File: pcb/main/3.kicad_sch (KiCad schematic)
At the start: 10 parts

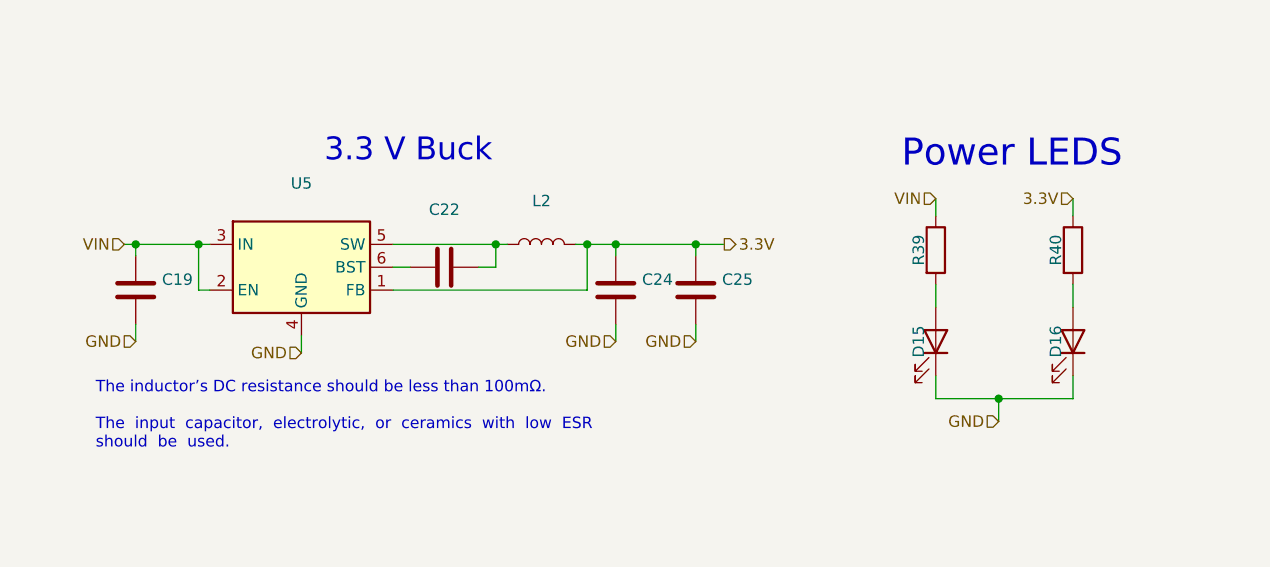
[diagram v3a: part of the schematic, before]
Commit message: feat: updated BOM
BOM ready to order in v0.2
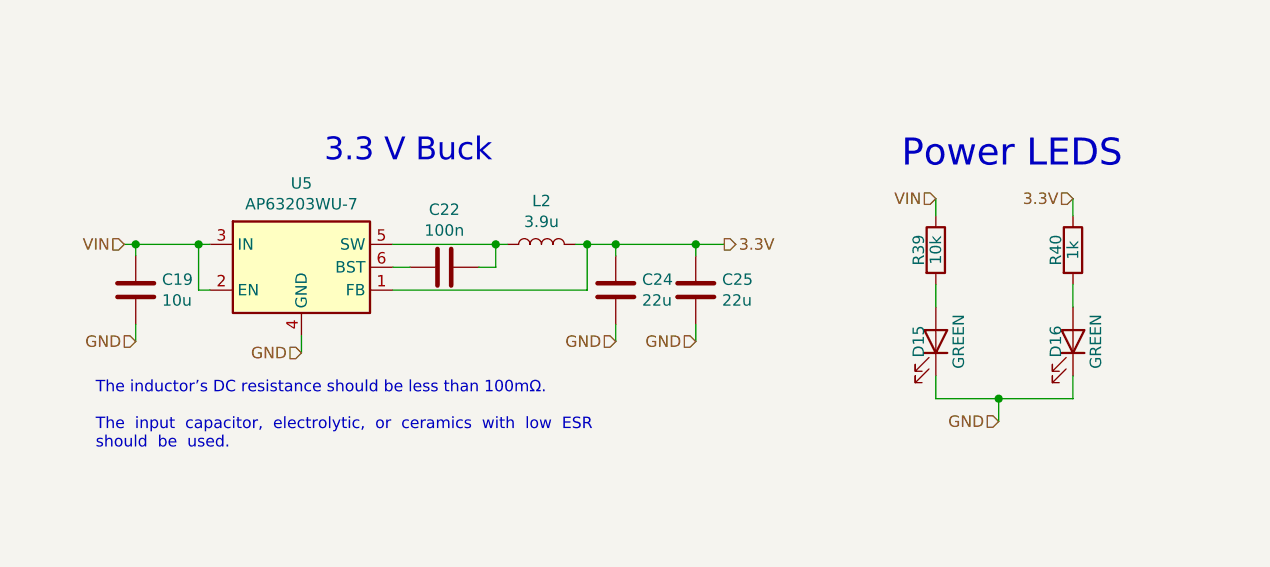
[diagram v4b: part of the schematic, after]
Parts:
- C19: value (none) -> 10u; footprint (none) -> Capacitor_SMD:C_0805_2012Metric_Pad1.18x1.45mm_HandSolder; MFN Wurth Elektronik -> Samsung Electro-Mechanics; MFP 885012207072 -> CL21A106KOQNNNG; S1PL https://www.mouser.com/ProductDetail/Wurth-Elektronik/88501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 -> https://www.mouser.com/ProductDetail/Samsung-Electro-Mechan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; S1PN 710-885012207072 -> 187-CL21A106KOQNNNG
- C22: value (none) -> 100n; footprint (none) -> Capacitor_SMD:C_0805_2012Metric_Pad1.18x1.45mm_HandSolder
- C24, C25: value (none) -> 22u; footprint (none) -> Capacitor_SMD:C_0805_2012Metric_Pad1.15x1.40mm_HandSolder
- D15, D16: value (none) -> GREEN; footprint (none) -> LED_SMD:LED_0805_2012Metric_Pad1.15x1.40mm_HandSolder
- L2: value (none) -> 3.9u; footprint (none) -> Inductor_SMD:L_Taiyo-Yuden_NR-24xx_HandSoldering
- R39: value (none) -> 10k; footprint (none) -> Resistor_SMD:R_0805_2012Metric_Pad1.20x1.40mm_HandSolder
- R40: value (none) -> 1k; footprint (none) -> Resistor_SMD:R_0805_2012Metric_Pad1.15x1.40mm_HandSolder
- U5: value (none) -> AP63203WU-7; footprint (none) -> Package_TO_SOT_SMD:TSOT-23-6
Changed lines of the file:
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@@
     (in_bom yes) (on_board yes)
     (property "Reference" "R39" (id 0) (at 172.085 95.885 90))
-    (property "Value" "" (id 1) (at 173.99 95.885 90))
-    (property "Footprint" "" (id 2) (at 172.212 95.885 90)
+    (property "Value" "10k" (id 1) (at 173.99 95.885 90))
+    (property "Footprint" "Resistor_SMD:R_0805_2012Metric_Pad1.20x1.40mm_HandSolder" (id 2) (at 172.212 95.885 90)
       (effects (font (size 1.27 1.27)) hide)
     )
@@
     (in_bom yes) (on_board yes)
     (property "Reference" "R40" (id 0) (at 187.325 95.885 90))
-    (property "Value" "" (id 1) (at 189.23 95.885 90))
-    (property "Footprint" "" (id 2) (at 187.452 95.885 90)
+    (property "Value" "1k" (id 1) (at 189.23 95.885 90))
+    (property "Footprint" "Resistor_SMD:R_0805_2012Metric_Pad1.15x1.40mm_HandSolder" (id 2) (at 187.452 95.885 90)
       (effects (font (size 1.27 1.27)) hide)
     )
@@
     (in_bom yes) (on_board yes)
     (property "Reference" "D15" (id 0) (at 172.085 106.045 0))
-    (property "Value" "" (id 1) (at 176.53 106.045 0))
-    (property "Footprint" "" (id 2) (at 173.99 106.045 0)
+    (property "Value" "GREEN" (id 1) (at 176.53 106.045 0))
+    (property "Footprint" "LED_SMD:LED_0805_2012Metric_Pad1.15x1.40mm_HandSolder" (id 2) (at 173.99 106.045 0)
       (effects (font (size 1.27 1.27)) hide)
     )
@@
     (in_bom yes) (on_board yes)
     (property "Reference" "D16" (id 0) (at 187.325 106.045 0))
-    (property "Value" "" (id 1) (at 191.77 106.045 0))
-    (property "Footprint" "" (id 2) (at 189.23 106.045 0)
+    (property "Value" "GREEN" (id 1) (at 191.77 106.045 0))
+    (property "Footprint" "LED_SMD:LED_0805_2012Metric_Pad1.15x1.40mm_HandSolder" (id 2) (at 189.23 106.045 0)
       (effects (font (size 1.27 1.27)) hide)
     )
@@
     (in_bom yes) (on_board yes)
     (property "Reference" "U5" (id 0) (at 103.505 88.4682 0))
-    (property "Value" "" (id 1) (at 103.505 90.7796 0))
-    (property "Footprint" "" (id 2) (at 103.505 120.65 0)
+    (property "Value" "AP63203WU-7" (id 1) (at 103.505 90.7796 0))
+    (property "Footprint" "Package_TO_SOT_SMD:TSOT-23-6" (id 2) (at 103.505 120.65 0)
       (effects (font (size 1.27 1.27)) hide)
     )
@@
       (effects (font (size 1.27 1.27)) (justify left))
     )
-    (property "Value" "" (id 1) (at 88.011 101.473 0)
+    (property "Value" "10u" (id 1) (at 88.011 101.473 0)
       (effects (font (size 1.27 1.27)) (justify left))
     )
-    (property "Footprint" "" (id 2) (at 86.0552 104.14 0)
-      (effects (font (size 1.27 1.27)) hide)
-    )
-    (property "Datasheet" "https://www.mouser.com/datasheet/2/445/885012207072-1727745.pdf" (id 3) (at 85.09 100.33 0)
-      (effects (font (size 1.27 1.27)) hide)
-    )
-    (property "Description" "Multilayer Ceramic Capacitors MLCC - SMD/SMT WCAP-CSGP 0.1uF 0805 10% 25V MLCC " (id 4) (at 85.09 100.33 0)
-      (effects (font (size 1.27 1.27)) hide)
-    )
-    (property "MFN" "Wurth Elektronik " (id 5) (at 85.09 100.33 0)
-      (effects (font (size 1.27 1.27)) hide)
-    )
-    (property "MFP" "885012207072" (id 6) (at 85.09 100.33 0)
-      (effects (font (size 1.27 1.27)) hide)
-    )
-    (property "S1PL" "https://www.mouser.com/ProductDetail/Wurth-Elektronik/885012207072?qs=0KOYDY2FL28rQMV4504TxA%3D%3D" (id 7) (at 85.09 100.33 0)
-      (effects (font (size 1.27 1.27)) hide)
-    )
-    (property "S1PN" "710-885012207072 " (id 8) (at 85.09 100.33 0)
+    (property "Footprint" "Capacitor_SMD:C_0805_2012Metric_Pad1.18x1.45mm_HandSolder" (id 2) (at 86.0552 104.14 0)
+      (effects (font (size 1.27 1.27)) hide)
+    )
+    (property "Datasheet" "https://www.mouser.com/datasheet/2/585/MLCC-1837944.pdf" (id 3) (at 85.09 100.33 0)
+      (effects (font (size 1.27 1.27)) hide)
+    )
+    (property "Description" "Capacitores cerámicos de capas múltiples (MLCC) - SMD/SMT 10uF+/-10% 16V X5R 2 0805 " (id 4) (at 85.09 100.33 0)
+      (effects (font (size 1.27 1.27)) hide)
+    )
+    (property "MFN" "Samsung Electro-Mechanics " (id 5) (at 85.09 100.33 0)
+      (effects (font (size 1.27 1.27)) hide)
+    )
+    (property "MFP" "CL21A106KOQNNNG " (id 6) (at 85.09 100.33 0)
+      (effects (font (size 1.27 1.27)) hide)
+    )
+    (property "S1PL" "https://www.mouser.com/ProductDetail/Samsung-Electro-Mechanics/CL21A106KOQNNNG?qs=hqM3L16%252BxlcMWI7QbqH0LA%3D%3D" (id 7) (at 85.09 100.33 0)
+      (effects (font (size 1.27 1.27)) hide)
+    )
+    (property "S1PN" "187-CL21A106KOQNNNG " (id 8) (at 85.09 100.33 0)
       (effects (font (size 1.27 1.27)) hide)
     )
@@
     (in_bom yes) (on_board yes)
     (property "Reference" "C22" (id 0) (at 119.38 91.3892 90))
-    (property "Value" "" (id 1) (at 119.38 93.7006 90))
-    (property "Footprint" "" (id 2) (at 115.57 98.7552 0)
+    (property "Value" "100n" (id 1) (at 119.38 93.7006 90))
+    (property "Footprint" "Capacitor_SMD:C_0805_2012Metric_Pad1.18x1.45mm_HandSolder" (id 2) (at 115.57 98.7552 0)
       (effects (font (size 1.27 1.27)) hide)
     )
@@
     (in_bom yes) (on_board yes)
     (property "Reference" "L2" (id 0) (at 130.175 90.424 90))
-    (property "Value" "" (id 1) (at 130.175 92.7354 90))
-    (property "Footprint" "" (id 2) (at 130.175 95.25 0)
+    (property "Value" "3.9u" (id 1) (at 130.175 92.7354 90))
+    (property "Footprint" "Inductor_SMD:L_Taiyo-Yuden_NR-24xx_HandSoldering" (id 2) (at 130.175 95.25 0)
       (effects (font (size 1.27 1.27)) hide)
     )
@@
       (effects (font (size 1.27 1.27)) (justify right))
     )
-    (property "Value" "" (id 1) (at 141.351 101.473 0)
-      (effects (font (size 1.27 1.27)) (justify right))
-    )
-    (property "Footprint" "" (id 2) (at 137.4648 96.52 0)
+    (property "Value" "22u" (id 1) (at 141.351 101.473 0)
+      (effects (font (size 1.27 1.27)) (justify right))
+    )
+    (property "Footprint" "Capacitor_SMD:C_0805_2012Metric_Pad1.15x1.40mm_HandSolder" (id 2) (at 137.4648 96.52 0)
       (effects (font (size 1.27 1.27)) hide)
     )
@@
       (effects (font (size 1.27 1.27)) (justify right))
     )
-    (property "Value" "" (id 1) (at 150.241 101.473 0)
-      (effects (font (size 1.27 1.27)) (justify right))
-    )
-    (property "Footprint" "" (id 2) (at 146.3548 96.52 0)
-      (effects (font (size 1.27 1.27)) hide)
-    )
+    (property "Value" "22u" (id 1) (at 150.241 101.473 0)
+      (effects (font (size 1.27 1.27)) (justify right))
+    )
+    (property "Footprint" "Capacitor_SMD:C_0805_2012Metric_Pad1.15x1.40mm_HandSolder" (id 2) (at 146.3548 96.52 0)
+      (effects (font (size 1.27 1.27)) hide)
+    )
